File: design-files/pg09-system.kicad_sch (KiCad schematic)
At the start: 31 parts, among them J101 Front Panel, SW201 NMI, SW201 Reset, U101 MC6809E, U102 GAL22V10, U103 74AHCT245, U104 74AHCT245, U105 74AHCT245, U106 GAL22V10, U203 DS1813

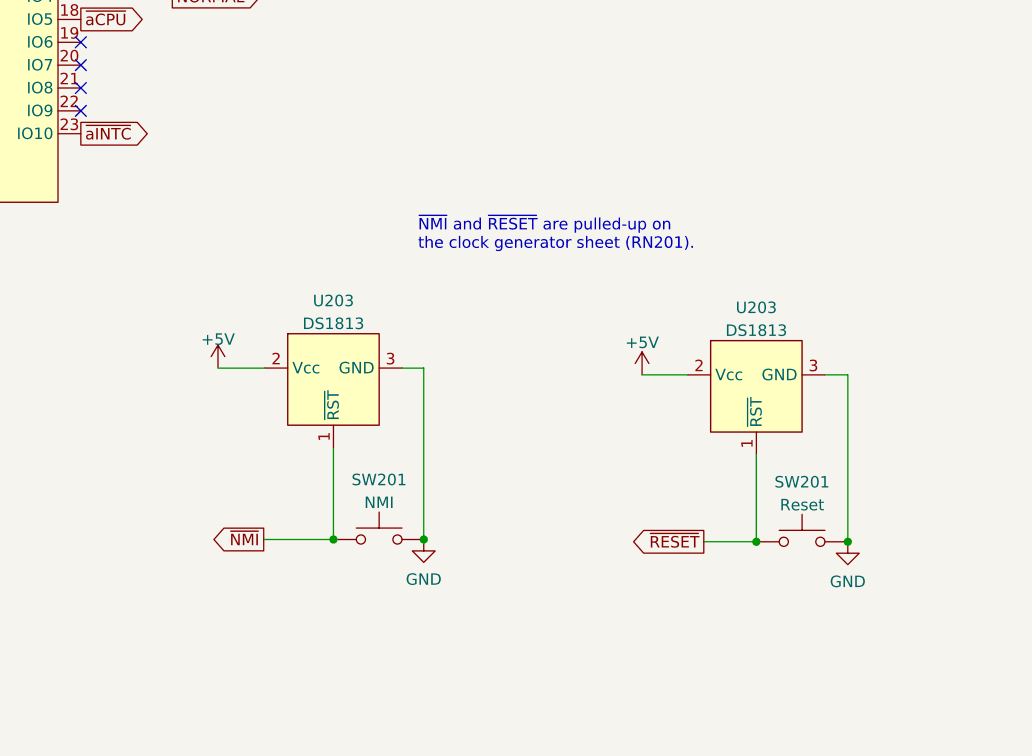
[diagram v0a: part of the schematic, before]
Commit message: Use an R-C circuit in front of the Vcc on /RESET's DS1813 in order to delay power-on-reset by ~0.75 seconds.
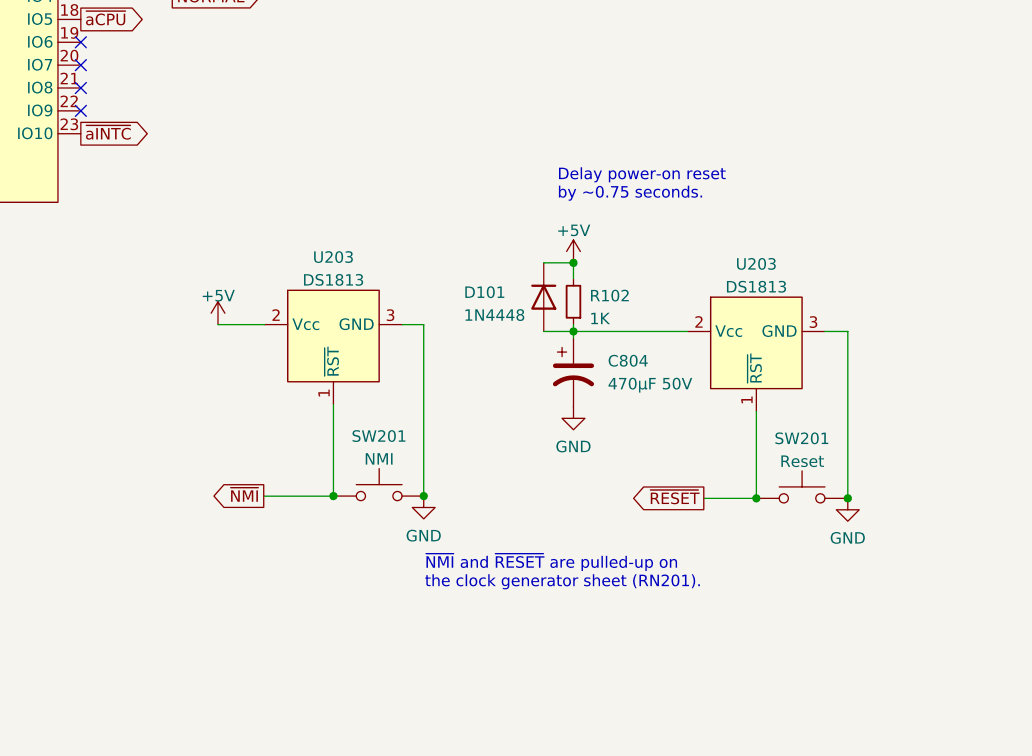
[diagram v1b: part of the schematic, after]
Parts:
- added C804: 470µF 50V, Capacitor_THT:CP_Radial_D12.5mm_P5.00mm, symbol Device:C_Polarized_US
- added D101: 1N4448, Diode_THT:D_DO-35_SOD27_P7.62mm_Horizontal, symbol Diode:1N4448
- added R102: 1K, Resistor_THT:R_Axial_DIN0207_L6.3mm_D2.5mm_P7.62mm_Horizontal, symbol Device:R_Small
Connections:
- net +5V: now also D101.1 (K), R102.2; no longer U203.2 (Vcc)
- net GND: now also C804.2
- new net: C804.1, D101.2 (A), R102.1, U203.2 (Vcc)
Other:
- note added: "Delay power-on reset by ~0.75 seconds."
- moved on the sheet: SW201, U203

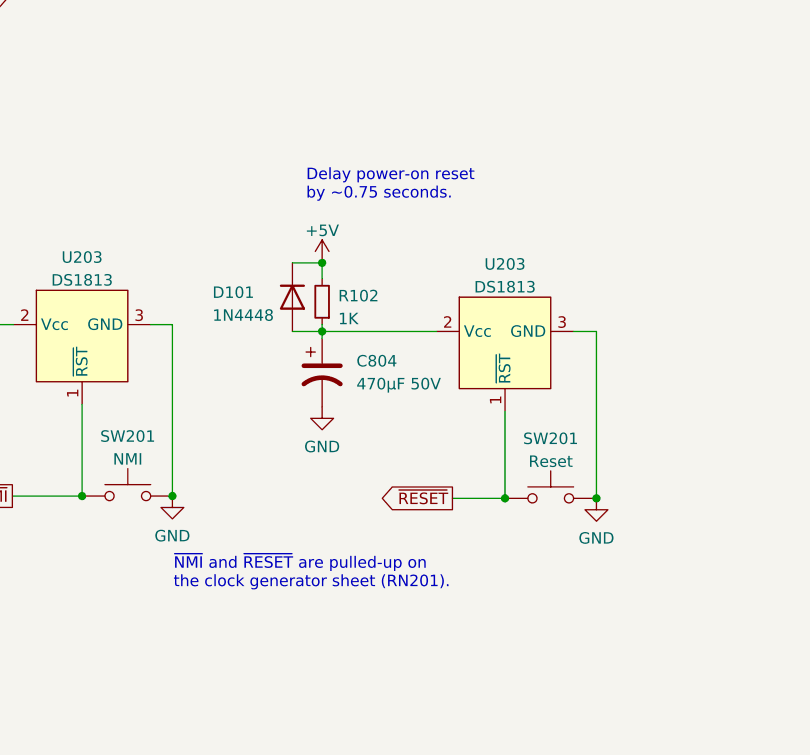
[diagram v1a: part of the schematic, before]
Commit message: Tweak the reset and NMI circuits -- no pull-ups on those signals needed; the DS1813 has us covered.  Add power-on-reset delay of ~0.5 seconds.
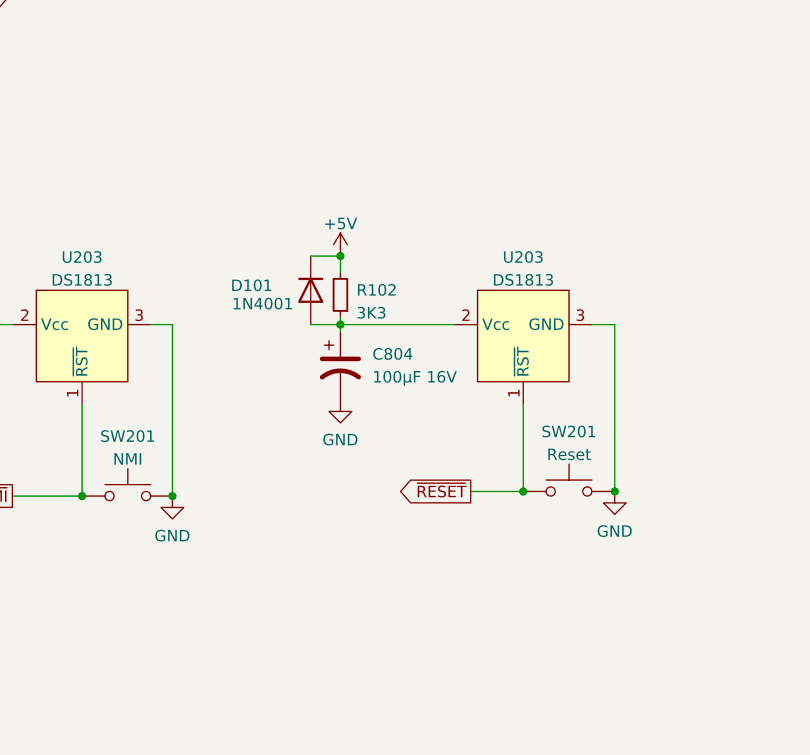
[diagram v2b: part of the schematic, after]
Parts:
- C804: value 470µF 50V -> 100µF 16V; footprint Capacitor_THT:CP_Radial_D12.5mm_P5.00mm -> Capacitor_THT:CP_Radial_D6.3mm_P2.50mm; Mouser 871-B41888C6477M -> 661-E-160L101MF11D
- D101: value 1N4448 -> 1N4001; footprint Diode_THT:D_DO-35_SOD27_P7.62mm_Horizontal -> Diode_THT:D_DO-41_SOD81_P10.16mm_Horizontal; symbol Diode:1N4448 -> Diode:1N4001
- R102: value 1K -> 3K3
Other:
- note removed: "Delay power-on reset by ~0.75 seconds."
- note removed: "~{NMI} and ~{RESET} are pulled-up on the clock generator sheet (RN201)."
- moved on the sheet: C804, D101, R102, SW201, U203
